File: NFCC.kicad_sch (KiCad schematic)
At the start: 67 parts, among them SW5 SW_Push, SW6 SW_SPDT, U10 IIS2MDCTR, U11 24CW1280T-I/OT, U12 BMI088, U7 BMP581, U8 W25N01GVZEIG, U9 PCA9685PW

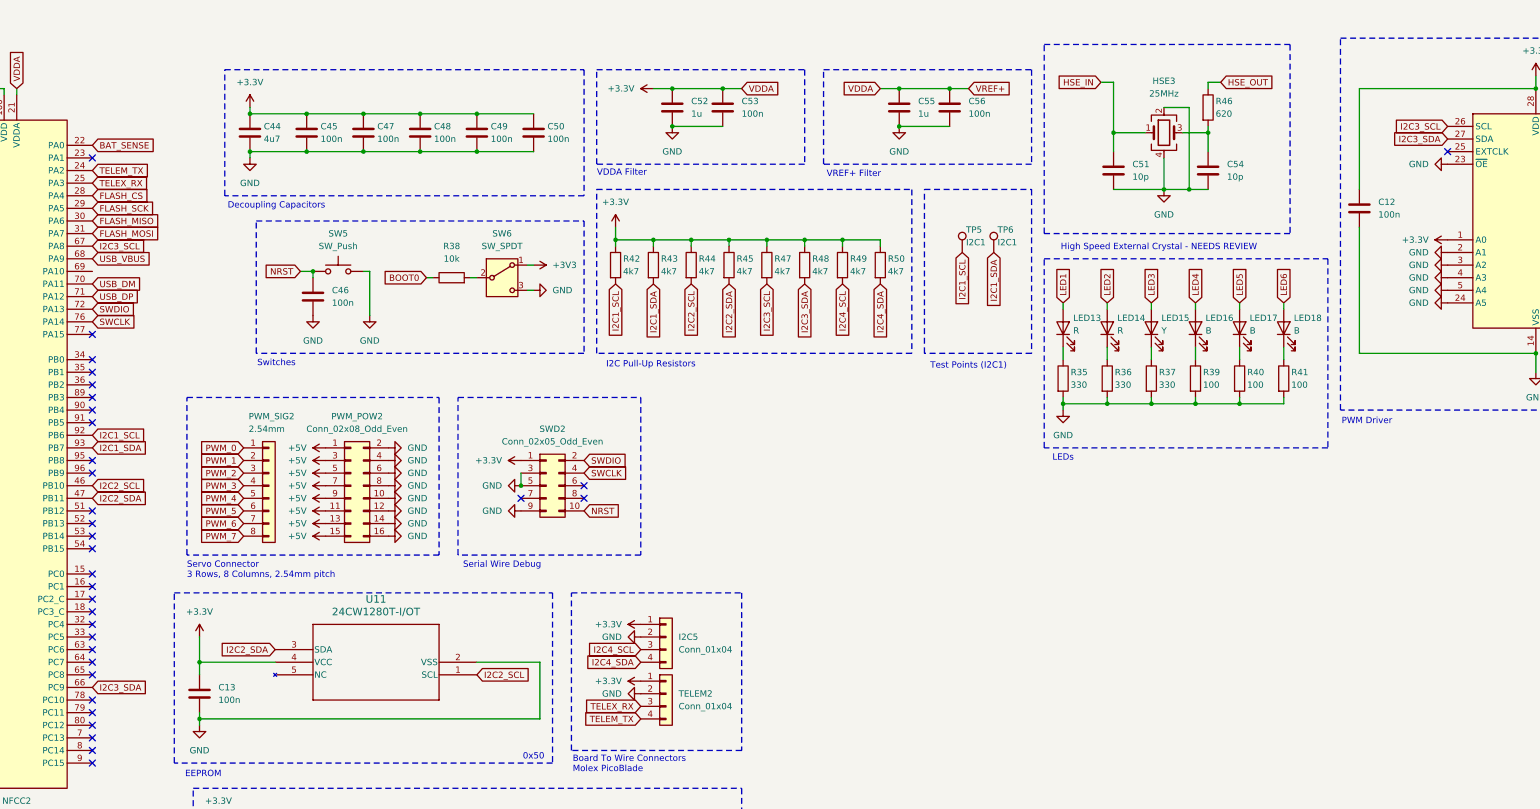
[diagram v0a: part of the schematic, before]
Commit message: Add files via upload
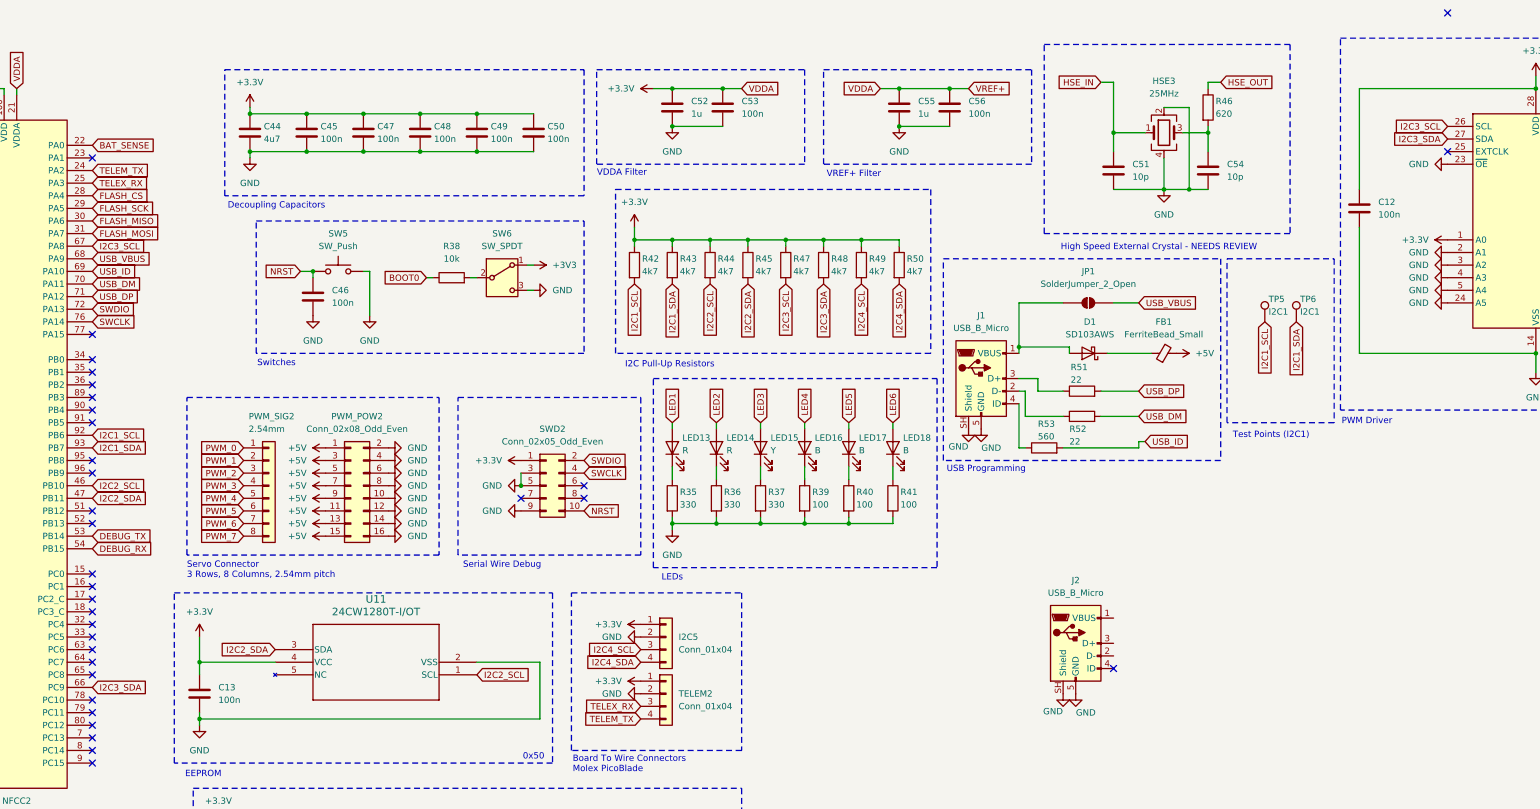
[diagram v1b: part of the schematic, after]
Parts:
- added D1: SD103AWS, Package_SON:WSON-8-1EP_6x5mm_P1.27mm_EP3.4x4mm, symbol Device:D_Schottky
- added FB1: FerriteBead_Small, symbol Device:FerriteBead_Small
- added J1, J2: USB_B_Micro, Package_DFN_QFN:WQFN-16-1EP_3x3mm_P0.5mm_EP1.75x1.75mm, symbol Connector:USB_B_Micro
- added JP1: SolderJumper_2_Open, Package_SON:WSON-8-1EP_6x5mm_P1.27mm_EP3.4x4mm, symbol Jumper:SolderJumper_2_Open
- added R51, R52: 22, symbol Device:R
- added R53: 560, symbol Device:R
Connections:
- net +5V: now also FB1.2
- net GND: now also J1.5 (GND), J1.SH (Shield), J2.5 (GND), J2.SH (Shield)
- net USB_DM: now also R52.2
- net USB_DP: now also R51.2
- net USB_VBUS: now also JP1.2 (B)
- net DEBUG_TX: now reaches NFCC2.53 (PB14)
- net DEBUG_RX: now reaches NFCC2.54 (PB15)
- net USB_ID: now reaches NFCC2.69 (PA10)
- net USB_ID: now also R53.2
- new net: J1.4 (ID), R53.1
- new net: D1.2 (A), J1.1 (VBUS), JP1.1 (A)
- new net: J1.2 (D-), R52.1
- new net: J1.3 (D+), R51.1
- new net: D1.1 (K), FB1.1
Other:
- note added: "USB Programming"
- moved on the sheet: LED13, LED14, LED15, LED16, LED17, LED18, R35, R36, R37, R39, R40, R41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

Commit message: Add files via upload
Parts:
- added C23, C24: 10u, Package_SO:TSSOP-28_4.4x9.7mm_P0.65mm, symbol Device:C
- added C57, C58, C59, C61: 100n, symbol Device:C
- added C60: 10u, symbol Device:C
- added C62, C63: 22u, symbol Device:C
- added D2: SD103AWS, Package_SON:WSON-8-1EP_6x5mm_P1.27mm_EP3.4x4mm, symbol Device:D_Schottky
- added D3, D4: G, Package_SO:SOIC-8_3.9x4.9mm_P1.27mm, symbol Device:LED
- added FB2: FerriteBead_Small, symbol Device:FerriteBead_Small
- added J3: LiPo Battery, symbol Connector_Generic:Conn_01x02
- added L1: 4.7u, Package_TO_SOT_SMD:SOT-23-6, symbol Device:L
- added R1: 100k, Package_DIP:DIP-8_W7.62mm, symbol Device:R
- added R2: 47k, Package_DIP:DIP-8_W7.62mm, symbol Device:R
- added R3: 52.3k, Package_DIP:DIP-8_W7.62mm, symbol Device:R
- added R54: 560, symbol Device:R
- added R55: 240, symbol Device:R
- added R6, R7: 10k, Package_DIP:DIP-8_W7.62mm, symbol Device:R
- added U1: CH330N, Package_SO:SOIC-8_3.9x4.9mm_P1.27mm, symbol Interface_USB:CH330N
- added U2: TPS54302, Package_TO_SOT_SMD:SOT-23-6, symbol Regulator_Switching:TPS54302
- added U3: LD39200PU33R, SON_DFN6_3X3_STM, symbol 2026-09-15_06-05-24:LD39200PU33R
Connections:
- net +3.3V: now also C24.1, D4.2 (A), U3.1 (OUT), U3.2 (ADJ/SENSE)
- net +5V: now also C23.1, C62.1, C63.1, FB2.2, L1.2, R3.2, U3.5 (EN), U3.6 (IN)
- net BAT_SENSE: now also C59.1, R1.2, R2.1
- net DEBUG_RX: now also U1.6 (TXD)
- net DEBUG_TX: now also U1.7 (RXD)
- net GND: now also C23.2, C24.2, C57.2, C58.2, C59.2, C60.2, C62.2, C63.2, J3.1 (Pin_1), R2.2, R54.1, R55.1, R6.1, U1.3 (GND), U2.1 (GND), U3.3 (GND), U3.7 (GND)
- net at J2.1 (VBUS): now also C58.1, D2.2 (A), D3.2 (A), U1.5 (VCC)
- net at J2.2 (D-): now also U1.2 (UD-)
- net at J2.3 (D+): now also U1.1 (UD+)
- net TELEX_RX renamed TELEM_RX
- new net: D2.1 (K), FB2.1
- new net: D3.1 (K), R54.2
- new net: R7.1, U2.3 (VIN)
- new net: C61.2, L1.1, U2.2 (SW)
- new net: R3.1, R6.2, U2.4 (FB)
- new net: C61.1, U2.6 (BOOT)
- new net: C57.1, U1.8 (V3)
- new net: D4.1 (K), R55.2
- new net VBAT: C60.1, J3.2 (Pin_2), R1.1, R7.2, U2.5 (EN)
- no-connect marks 66 -> 68
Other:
- note added: "3.3V Regulator"
- note added: "5V Buck Converter"
- note added: "LiPo Battery Input"
- note added: "USB Debug"
- moved on the sheet: C12, C16, C18, C19, C51, C52, C53, C54, C55, C56, HSE3, J2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
